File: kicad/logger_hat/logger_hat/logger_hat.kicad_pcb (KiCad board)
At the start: 2 copper layers, 190.5 x 73.7 mm, 22 parts, among them J1 CO2_sensor_conn, J10 Conn_01x04_Pin, J2 5V_sensor_conn, J3 CH4_Sensor_conn, J4 Reed_switch_conn, J5 PWM_output_1, J6 log_switch_conn, J7 PWM_output_2

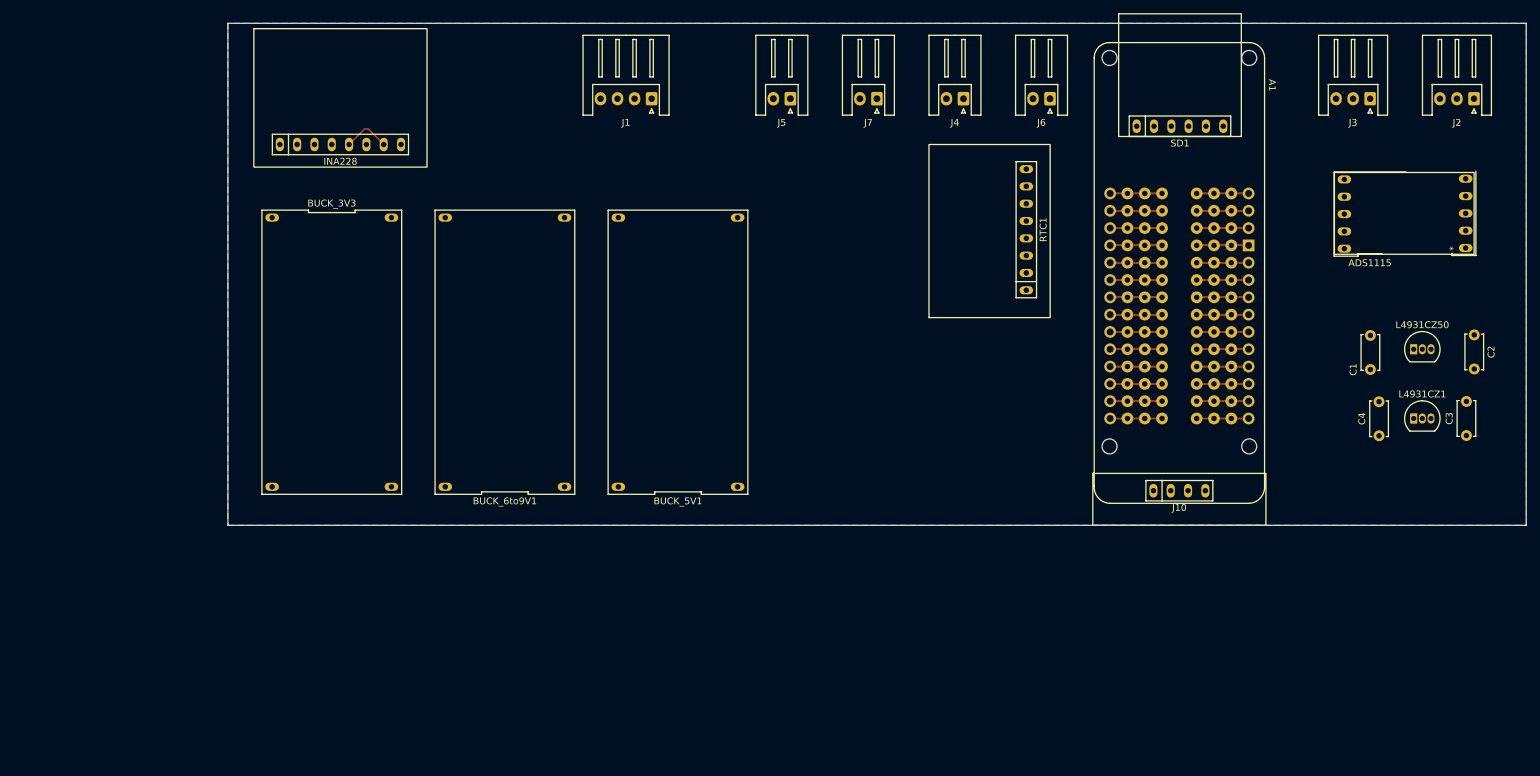
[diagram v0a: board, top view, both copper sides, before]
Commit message: Read work log
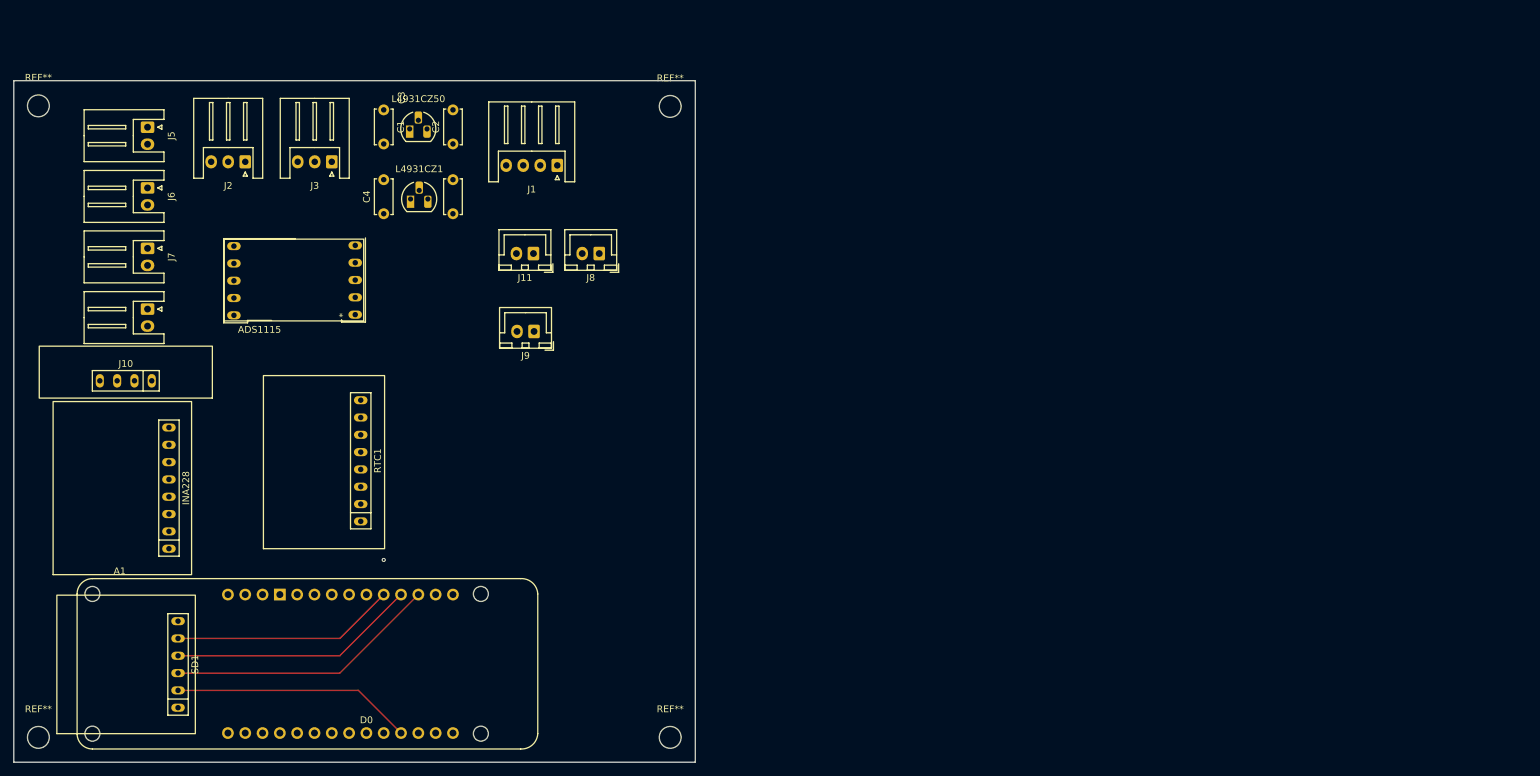
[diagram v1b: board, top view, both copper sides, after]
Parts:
- removed BUCK_3V3, BUCK_5V1, BUCK_6to9V1: ~, new_library:LM2596_module_amazon
- added J11: 5V6_IN, Connector_JST:JST_XH_B2B-XH-A_1x02_P2.50mm_Vertical, F.Cu at (103.3, 74.4)
- added J8: 7V_IN, Connector_JST:JST_XH_B2B-XH-A_1x02_P2.50mm_Vertical, F.Cu at (112.9, 74.4)
- added J9: 3V3_IN, Connector_JST:JST_XH_B2B-XH-A_1x02_P2.50mm_Vertical, F.Cu at (103.3, 85.9)
- added REF**: MountingHole_3.2mm_M3, MountingHole:MountingHole_3.2mm_M3, F.Cu at (123.3, 52.8)
- added REF**: MountingHole_3.2mm_M3, MountingHole:MountingHole_3.2mm_M3, F.Cu at (123.3, 145.4)
- added REF**: MountingHole_3.2mm_M3, MountingHole:MountingHole_3.2mm_M3, F.Cu at (30.6, 145.4)
- added REF**: MountingHole_3.2mm_M3, MountingHole:MountingHole_3.2mm_M3, F.Cu at (30.6, 52.8)
- J2: value 5V_sensor_conn -> 3V3_sensor_conn
- J4: value Reed_switch_conn -> SW_RD
- J6: value log_switch_conn -> SW_LOG
- L4931CZ1, L4931CZ50: footprint Package_TO_SOT_THT:TO-92_Inline -> Package_TO_SOT_THT:TO-92_HandSolder
- moved A1 187.1 mm to (38.5, 124.4), turned to 0 degrees
- moved J2 180.5 mm to (61.0, 61.0)
- moved SD1 166.9 mm to (51.1, 134.7), turned to 90 degrees
- moved ADS1115 163.2 mm to (73.3, 78.3)
- moved J10 155.4 mm to (43.4, 93.1), turned to 180 degrees
- moved J3 152.6 mm to (73.7, 61.0)
- moved C2 152.5 mm to (91.4, 58.3), turned to 90 degrees
- moved C3 152.2 mm to (91.4, 68.6)
- moved L4931CZ50 150.8 mm to (85.1, 56.1)
- moved L4931CZ1 150.7 mm to (85.2, 66.4)
- moved C1 149.7 mm to (81.3, 53.3), turned to -90 degrees
- moved C4 149.6 mm to (81.3, 68.6)
- moved J6 133.1 mm to (46.6, 64.8), turned to -90 degrees
- moved J4 123.6 mm to (46.6, 82.6), turned to -90 degrees
- moved J7 109.3 mm to (46.6, 73.7), turned to -90 degrees
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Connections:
- RTC1 pad 1: unconnected-(RTC1-Vin-Pad1) -> /3V3
- RTC1 pad 2: unconnected-(RTC1-GND-Pad2) -> GND
- RTC1 pad 3: unconnected-(RTC1-SCL-Pad3) -> /SCL
- RTC1 pad 4: unconnected-(RTC1-SDA-Pad4) -> /SDA
- RTC1 pad 7: unconnected-(RTC1-SQW-Pad7) -> /D3
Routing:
- net /MOSI: track 0.00 -> 40.0 mm
- net /SCK: track 0.00 -> 36.4 mm
- net /D2: track 0.00 -> 35.3 mm
- net /MISO: track 0.00 -> 32.8 mm
- net /V_bat: track 6.95 -> 0.00 mm
- net /D3: vias 0 -> 1
- removed copper zone on B.Cu, net GND
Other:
- board size 190.5 x 73.7 mm -> 100 x 100 mm
